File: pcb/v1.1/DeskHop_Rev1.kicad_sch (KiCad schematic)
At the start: 20 parts, among them J1 Keyboard In, J2 Debug2, J3 Debug1, J4 Mouse In, U1 Pico Primary, U2 Pico Secondary, U3 TPD4E1U06DBVR, U4 ADuM1201BR, U5 TPD4E1U06DBVR

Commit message: update smd r/c to 1206 size
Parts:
- C1, C2, C3, C4: footprint Capacitor_SMD:C_0805_2012Metric -> Capacitor_SMD:C_1206_3216Metric_Pad1.33x1.80mm_HandSolder
- R1, R2, R3, R4: footprint Resistor_SMD:R_0805_2012Metric -> Resistor_SMD:R_1206_3216Metric_Pad1.30x1.75mm_HandSolder

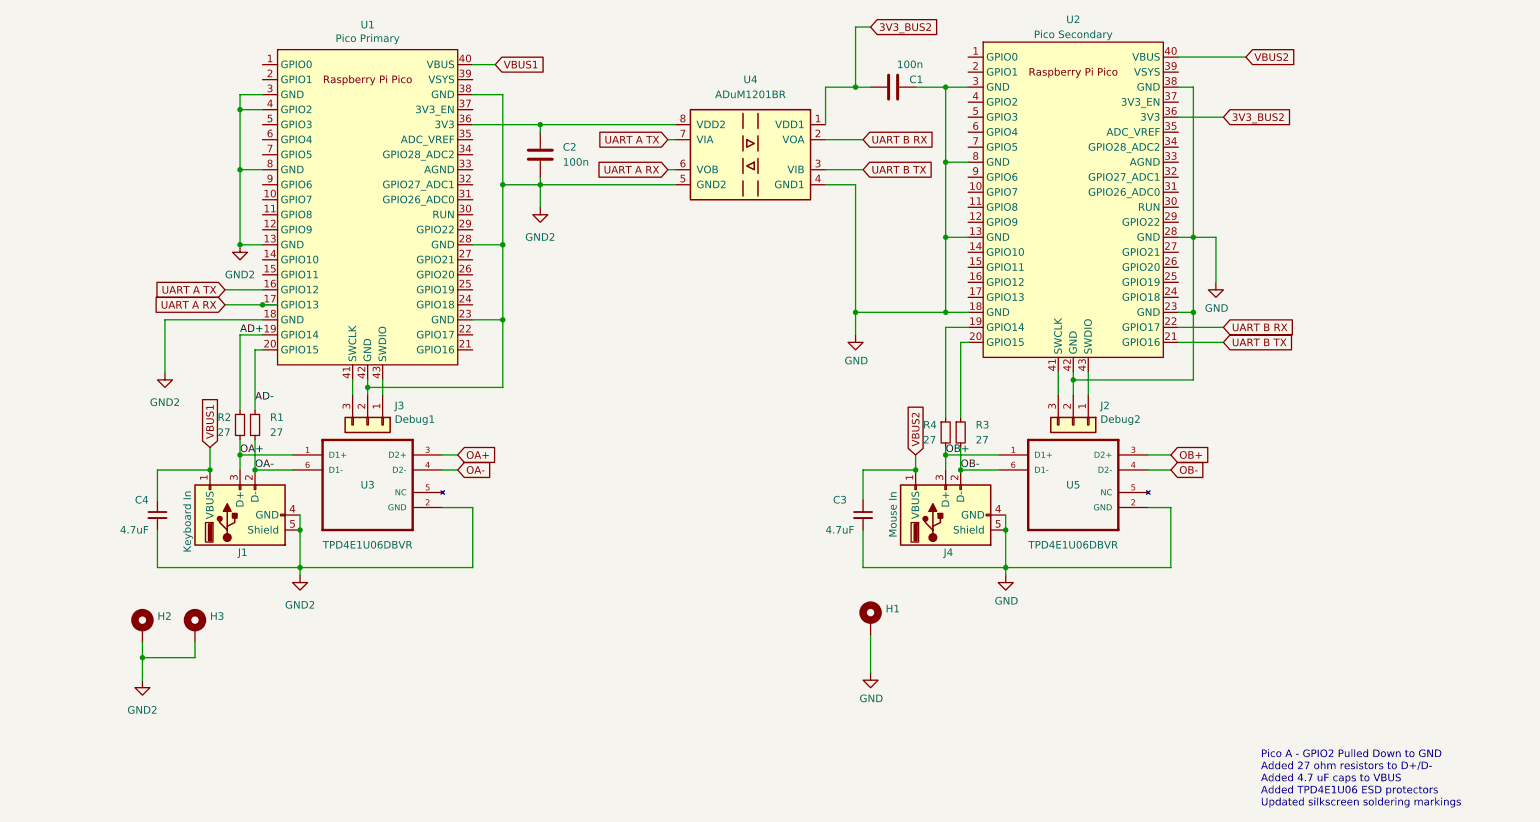
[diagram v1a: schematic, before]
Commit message: initial rework, connection to be reviewed
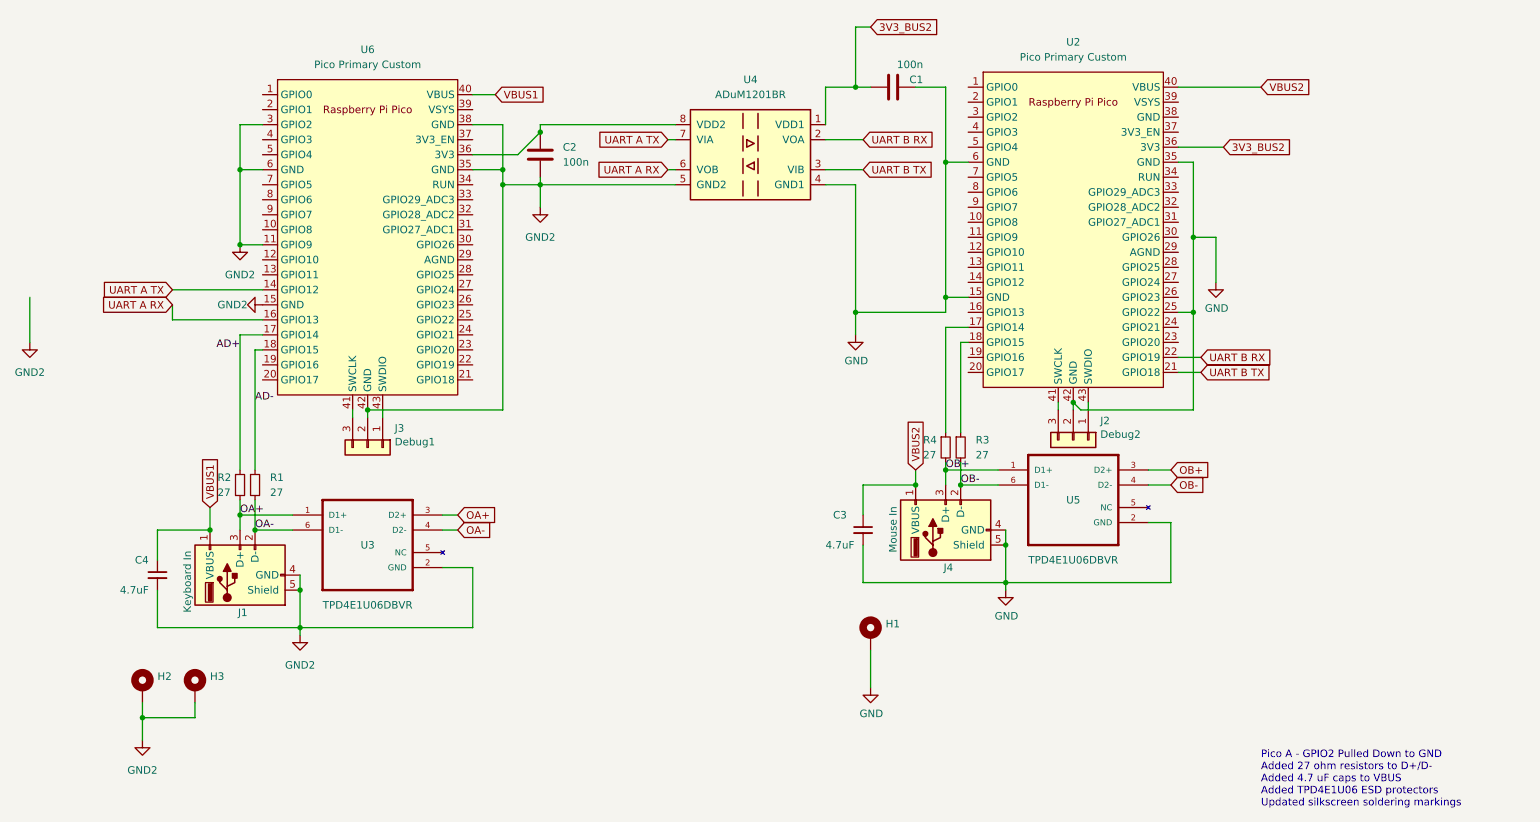
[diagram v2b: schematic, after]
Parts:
- removed U1: Pico Primary, MCU_RaspberryPi_and_Boards:RPi_Pico_SMD_TH, symbol MCU_RaspberryPi_and_Boards:Pico
- removed U2: Pico Secondary, MCU_RaspberryPi_and_Boards:RPi_Pico_SMD_TH, symbol MCU_RaspberryPi_and_Boards:Pico
- added U2, U6: Pico Primary Custom, RP2040:RPi_Pico_USBC_CUSTOM_SMD_TH, symbol Custom:Pico
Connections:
- net 3V3_BUS2: now also U2.36 (3V3)
- net AD+: now also U6.17 (GPIO14)
- net AD-: now also U6.18 (GPIO15)
- net GND: now also U2.15 (GND), U2.25 (GPIO22), U2.35 (GND), U2.42 (GND), U2.6 (GND)
- net GND2: now also U6.11 (GPIO9), U6.15 (GND), U6.3 (GPIO2), U6.35 (GND), U6.38 (GND), U6.42 (GND), U6.6 (GND)
- net UART A RX: now also U6.16 (GPIO13)
- net UART A TX: now also U6.14 (GPIO12)
- net UART B RX: now also U2.22 (GPIO19)
- net UART B TX: now also U2.21 (GPIO18)
- net VBUS1: now also U6.40 (VBUS)
- net VBUS2: now also U2.40 (VBUS)
- net at C2.1, U4.8 (VDD2): now also U6.36 (3V3)
- net at J3.3 (Pin_3): now also U6.41 (SWCLK)
- net at J3.1 (Pin_1): now also U6.43 (SWDIO)
- net at R3.1: now also U2.18 (GPIO15)
- net at J2.1 (Pin_1): now also U2.43 (SWDIO)
- net at J2.3 (Pin_3): now also U2.41 (SWCLK)
- net at R4.1: now also U2.17 (GPIO14)
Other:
- moved on the sheet: C3, C4, H1, H2, H3, J1, J2, J3, J4, R1, R2, R3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
